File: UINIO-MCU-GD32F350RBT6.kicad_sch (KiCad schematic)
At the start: 31 parts, among them J1 Conn_01x32_Male, J2 Conn_01x32_Male, J3 Conn_01x04_Male, SW1 BOOT0, SW2 NRST, U1 ME6211C33M5G-N, U2 GD32F350RBT6, Y1 32.768KHz, Y2 8MHz

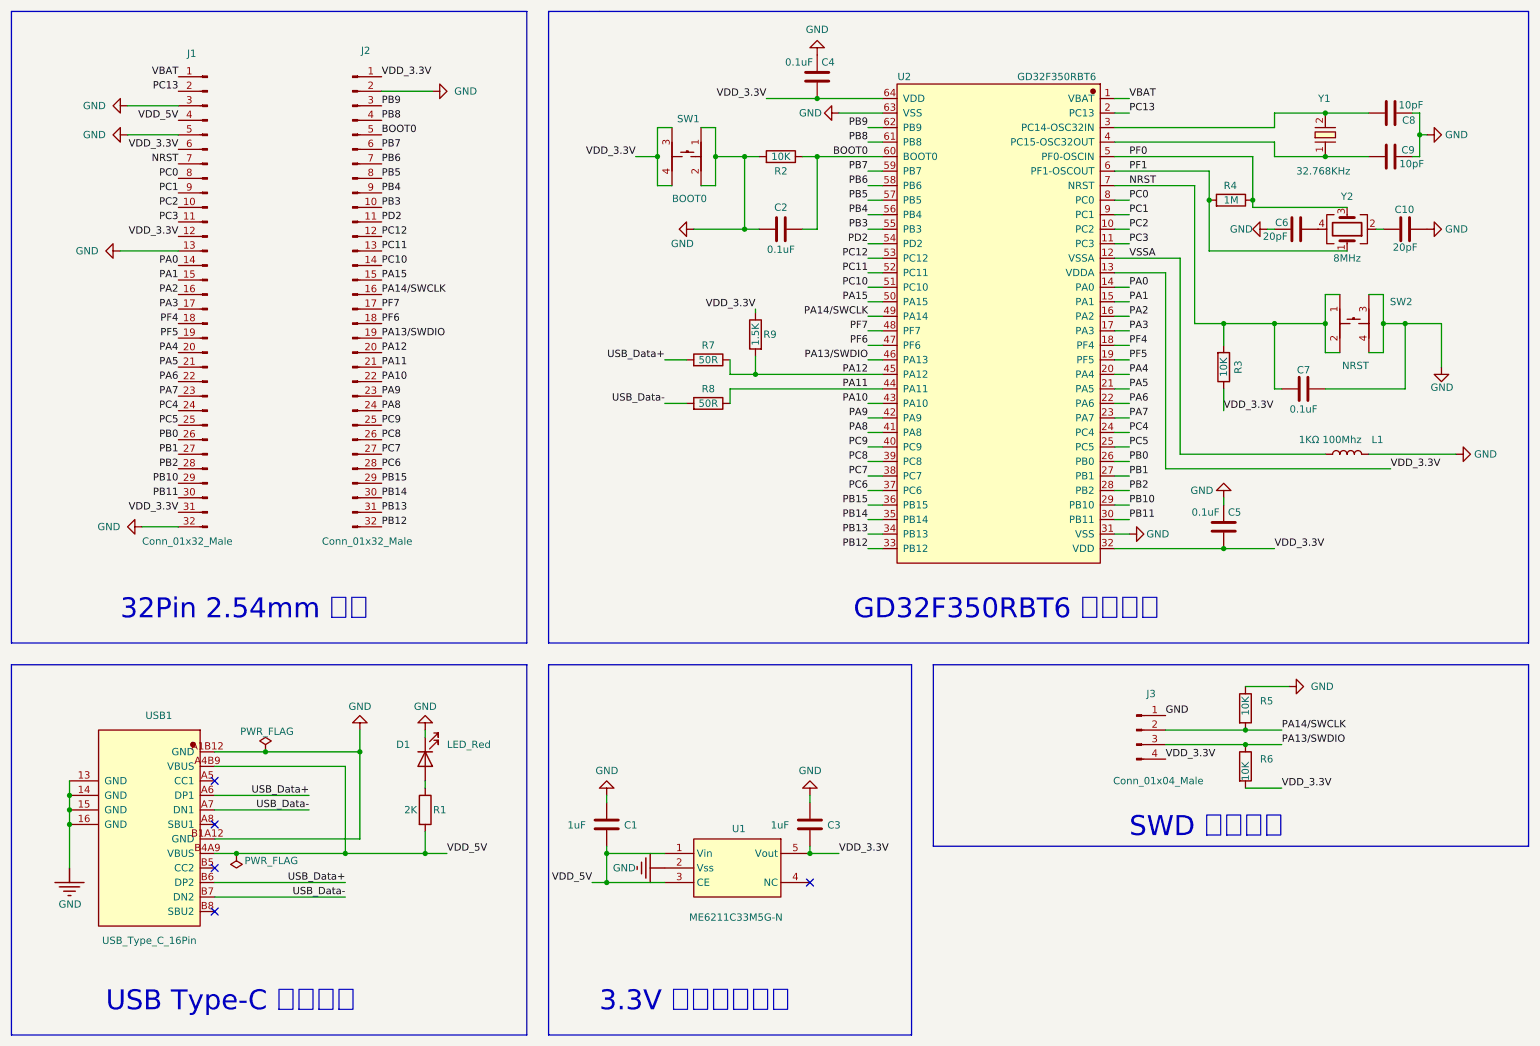
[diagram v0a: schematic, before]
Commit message: Release UINIO-MCU-GD32F350RBT6 version 1.0.0.
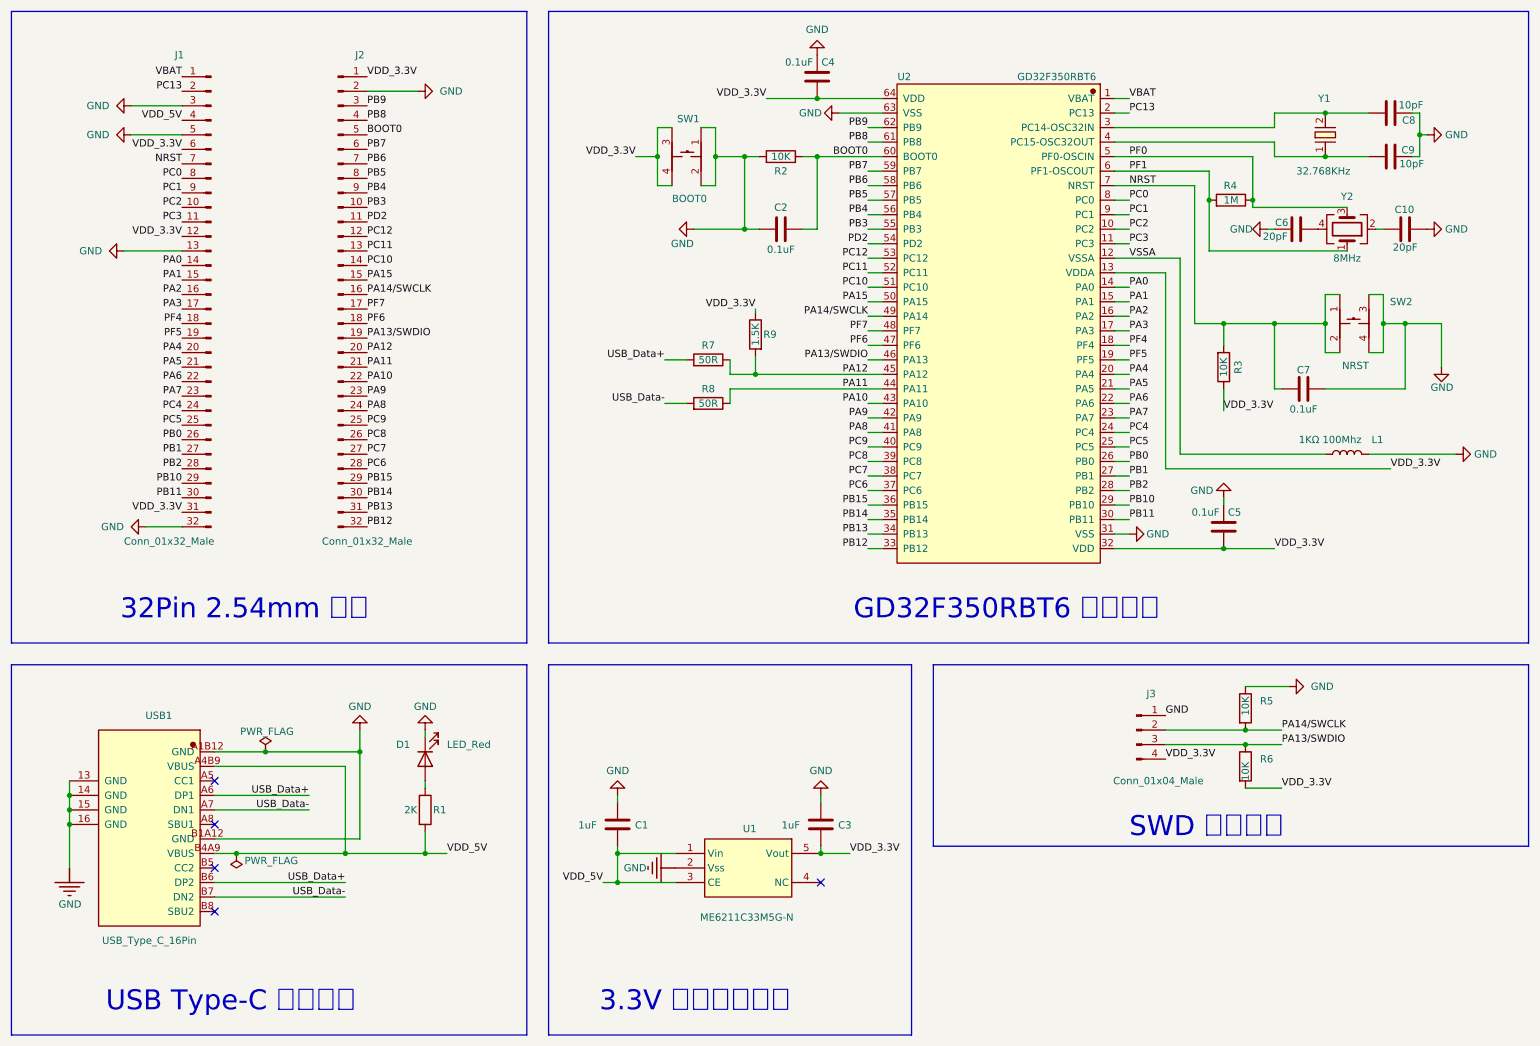
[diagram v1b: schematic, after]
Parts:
- J3: footprint Connector_PinHeader_2.54mm:PinHeader_1x04_P2.54mm_Vertical -> Connector_PinHeader_2.54mm:PinHeader_1x04_P2.54mm_Horizontal
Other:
- moved on the sheet: C1, C3, J1, J2, U1
